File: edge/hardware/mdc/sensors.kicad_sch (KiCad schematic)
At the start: 6 parts, among them U2 INMP441, U3 GY-906, U4 STEVAL-MKIGIBV2, U6 ACS712-30A

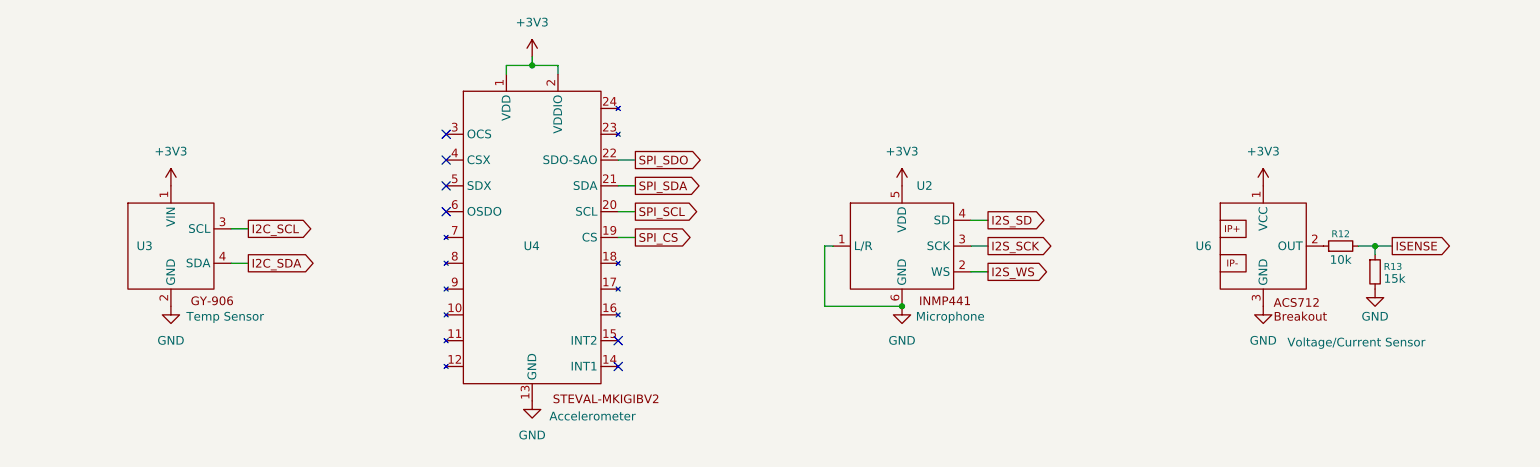
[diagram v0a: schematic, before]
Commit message: update rev3.0 schematic and layout
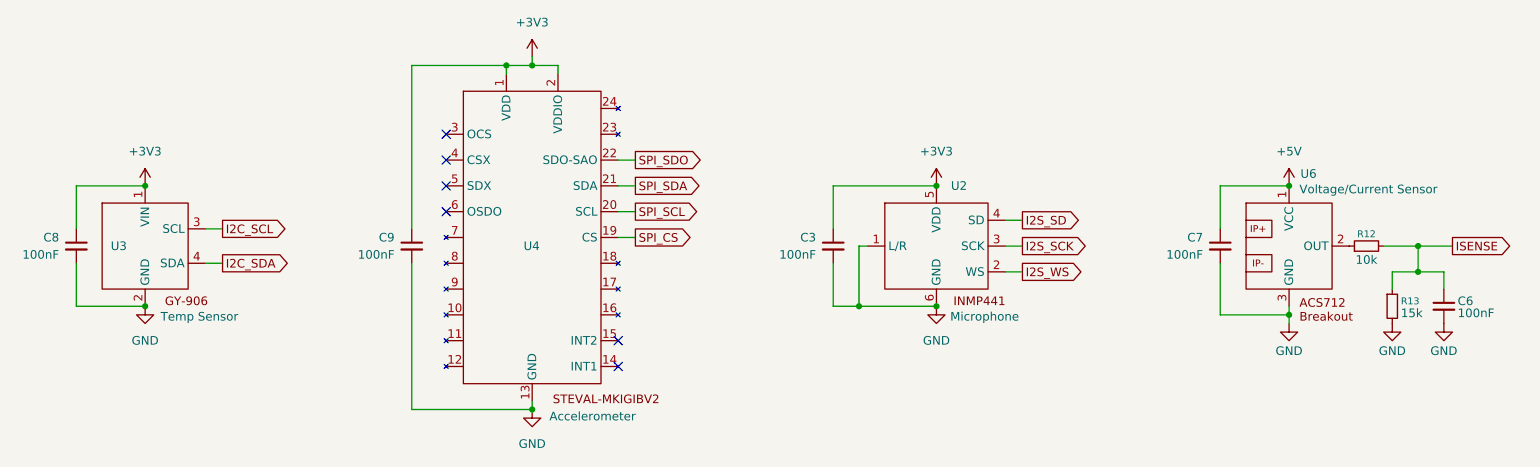
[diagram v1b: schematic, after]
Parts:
- added C3, C6, C7, C8, C9: 100nF, Capacitor_THT:C_Disc_D5.0mm_W2.5mm_P5.00mm, symbol Device:C_Small
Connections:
- net +3V3: now also C3.1, C8.1, C9.1; no longer U6.1 (VCC)
- net GND: now also C3.2, C6.2, C7.2, C8.2, C9.2
- net ISENSE: now also C6.1
- new net +5V: C7.1, U6.1 (VCC)
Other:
- moved on the sheet: R12, R13, U2, U3, U6
